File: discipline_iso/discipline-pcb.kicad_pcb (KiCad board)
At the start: 2 copper layers, 304.9 x 122.8 mm, 181 parts, among them J1 AVR-ISP-6, SW1 KEYSW, SW10 KEYSW, SW11 KEYSW, SW12 KEYSW, SW13 KEYSW, SW14 KEYSW, SW15 KEYSW, SW16 KEYSW, SW17 KEYSW, SW18 KEYSW, SW19 KEYSW, SW2 KEYSW, SW20 KEYSW, SW21 KEYSW, SW22 KEYSW, SW23 KEYSW, SW24 KEYSW, SW25 KEYSW, SW26 KEYSW, SW27 KEYSW, SW28 KEYSW, SW29 KEYSW, SW3 KEYSW, SW30 KEYSW, SW31 KEYSW, SW310 KEYSW, SW32 KEYSW, SW33 KEYSW, SW34 KEYSW, SW35 KEYSW, SW36 KEYSW, SW37 KEYSW, SW38 KEYSW, SW39 KEYSW, SW4 KEYSW, SW40 KEYSW, SW41 KEYSW, SW42 KEYSW, SW43 KEYSW, SW44 KEYSW, SW45 KEYSW, SW46 KEYSW, SW47 KEYSW, SW48 KEYSW, SW49 KEYSW, SW5 KEYSW, SW50 KEYSW, SW51 KEYSW, SW52 KEYSW, SW53 KEYSW, SW54 KEYSW, SW55 KEYSW, SW56 KEYSW, SW57 KEYSW, SW58 KEYSW, SW59 KEYSW, SW590 KEYSW, SW6 KEYSW, SW60 KEYSW, SW61 KEYSW, SW610 KEYSW, SW62 KEYSW, SW620 KEYSW, SW63 KEYSW, SW630 KEYSW, SW64 KEYSW, SW640 KEYSW, SW65 KEYSW, SW66 KEYSW, SW67 KEYSW, SW68 KEYSW, SW69 KEYSW, SW7 KEYSW, SW8 KEYSW, SW9 KEYSW, U1 ATmega32A-PU, Y1 Crystal

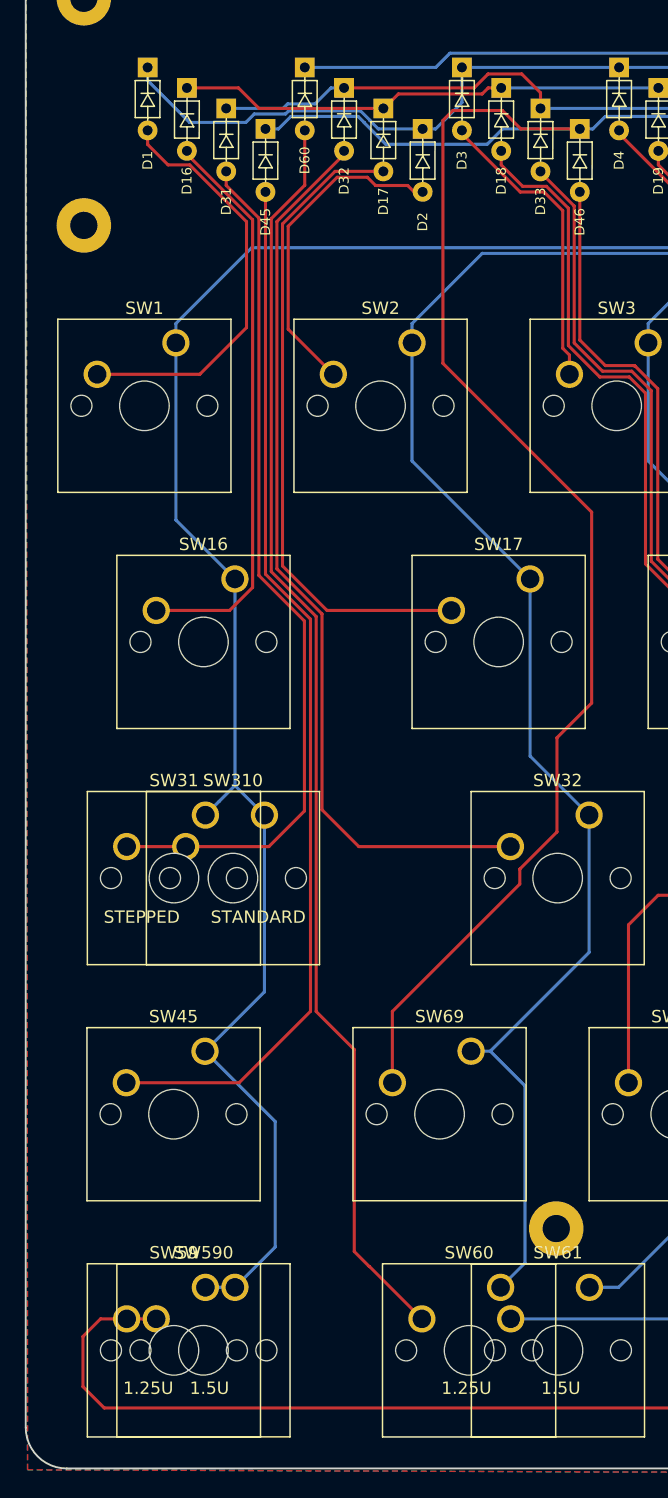
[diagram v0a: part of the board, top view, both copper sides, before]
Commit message: Add files via upload
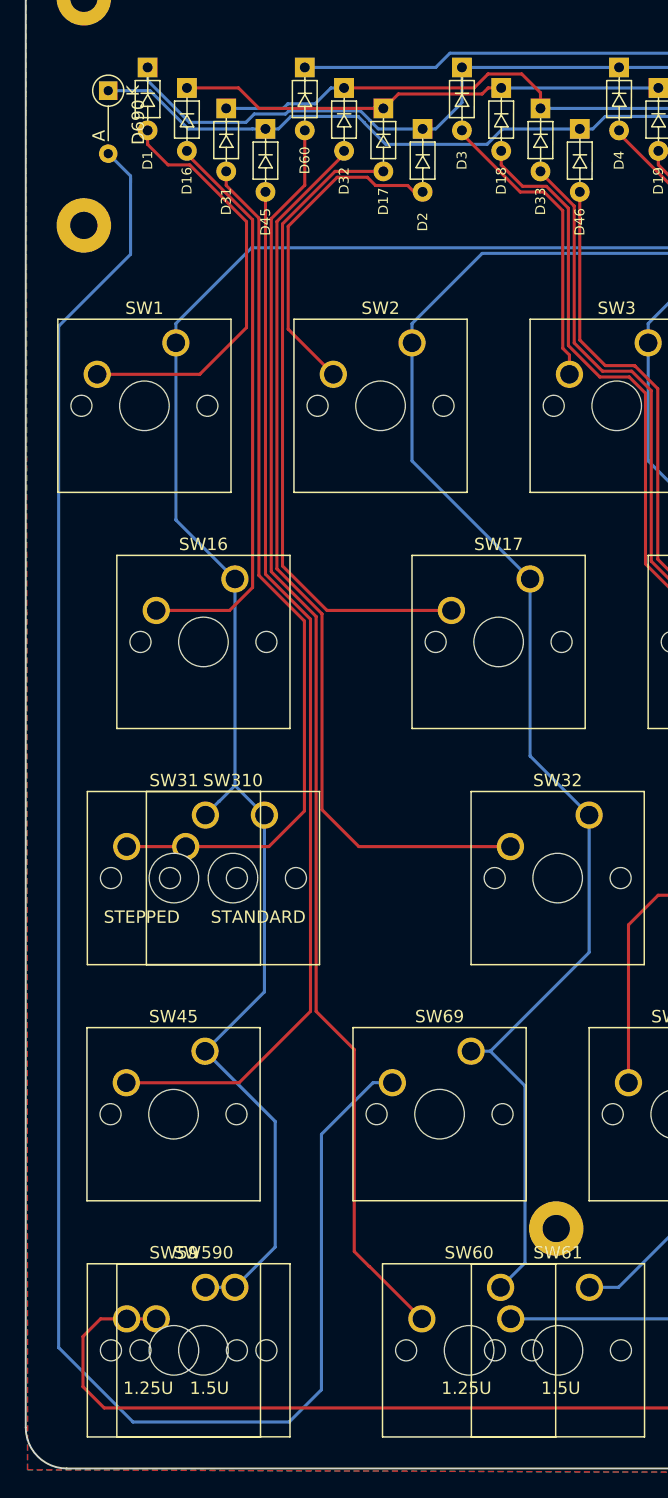
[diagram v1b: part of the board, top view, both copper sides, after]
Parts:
- added D690: , Diode_THT:D_DO-34_SOD68_P5.08mm_Vertical_AnodeUp, F.Cu at (67.2, 64.6)
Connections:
- SW69 pad 2: row3 -> Net-(D690-Pad2)
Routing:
- net Net-(D690-Pad2): track 0.00 -> 152.6 mm
- net row3: track 388.2 -> 300.9 mm
